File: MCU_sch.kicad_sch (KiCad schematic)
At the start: 10 parts

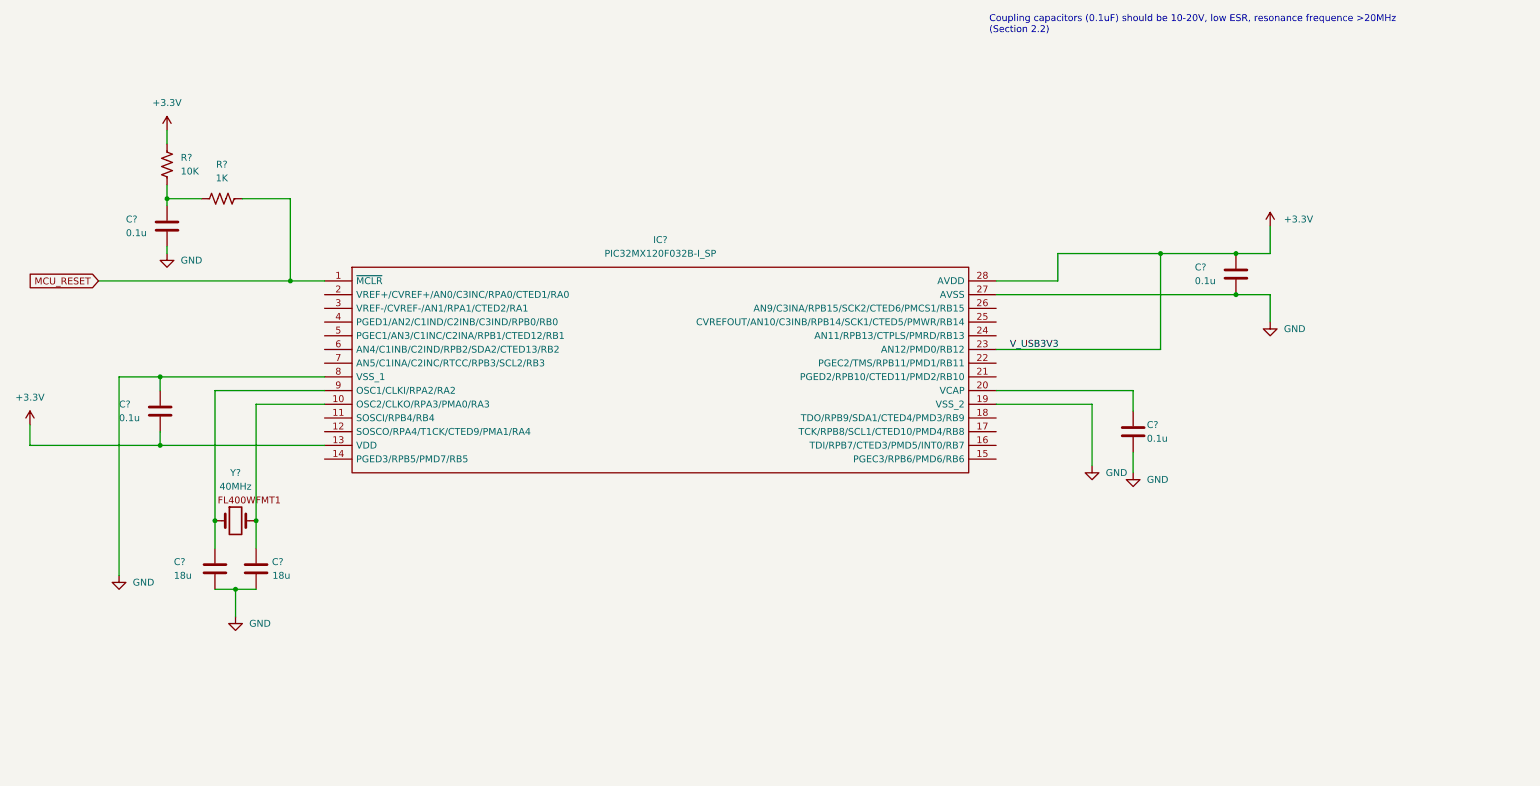
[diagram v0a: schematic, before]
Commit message: WIP output stage
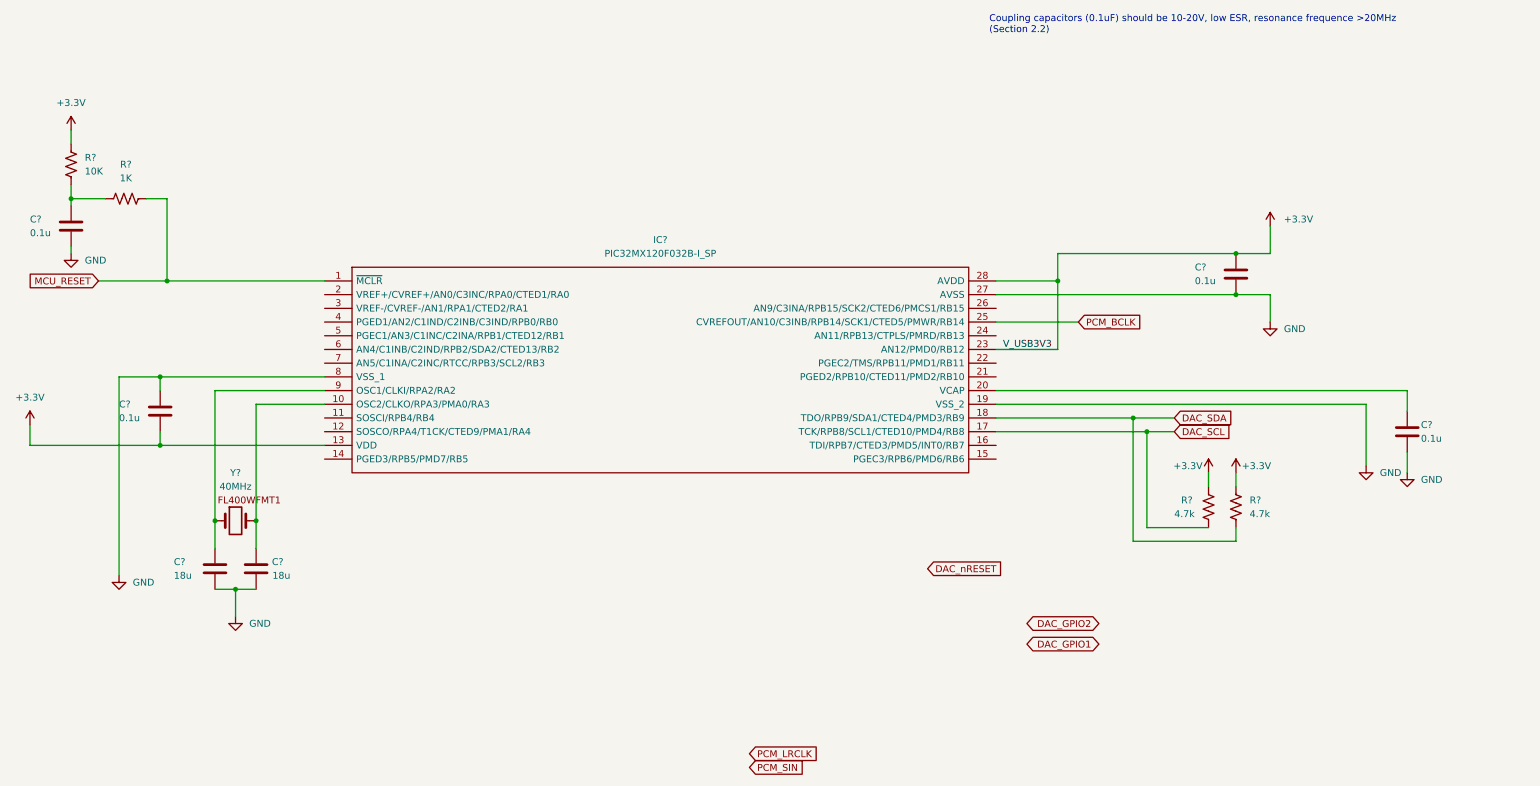
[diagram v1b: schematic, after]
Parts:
- added R? (x2): 4.7k, symbol Device:R_US
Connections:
- net +3V3: now also R?.1, R?.1
- net DAC_SCL: now reaches IC?.17 (TCK/RPB8/SCL1/CTED10/PMD4/RB8)
- net DAC_SCL: now also R?.2
- net DAC_SDA: now reaches IC?.18 (TDO/RPB9/SDA1/CTED4/PMD3/RB9)
- net DAC_SDA: now also R?.2
- net PCM_BCLK: now reaches IC?.25 (CVREFOUT/AN10/C3INB/RPB14/SCK1/CTED5/PMWR/RB14)
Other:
- moved on the sheet: C?, R?
